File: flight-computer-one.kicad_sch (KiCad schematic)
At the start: 10 parts, among them J1 LEFT_BANK, J2 RIGHT_BANK

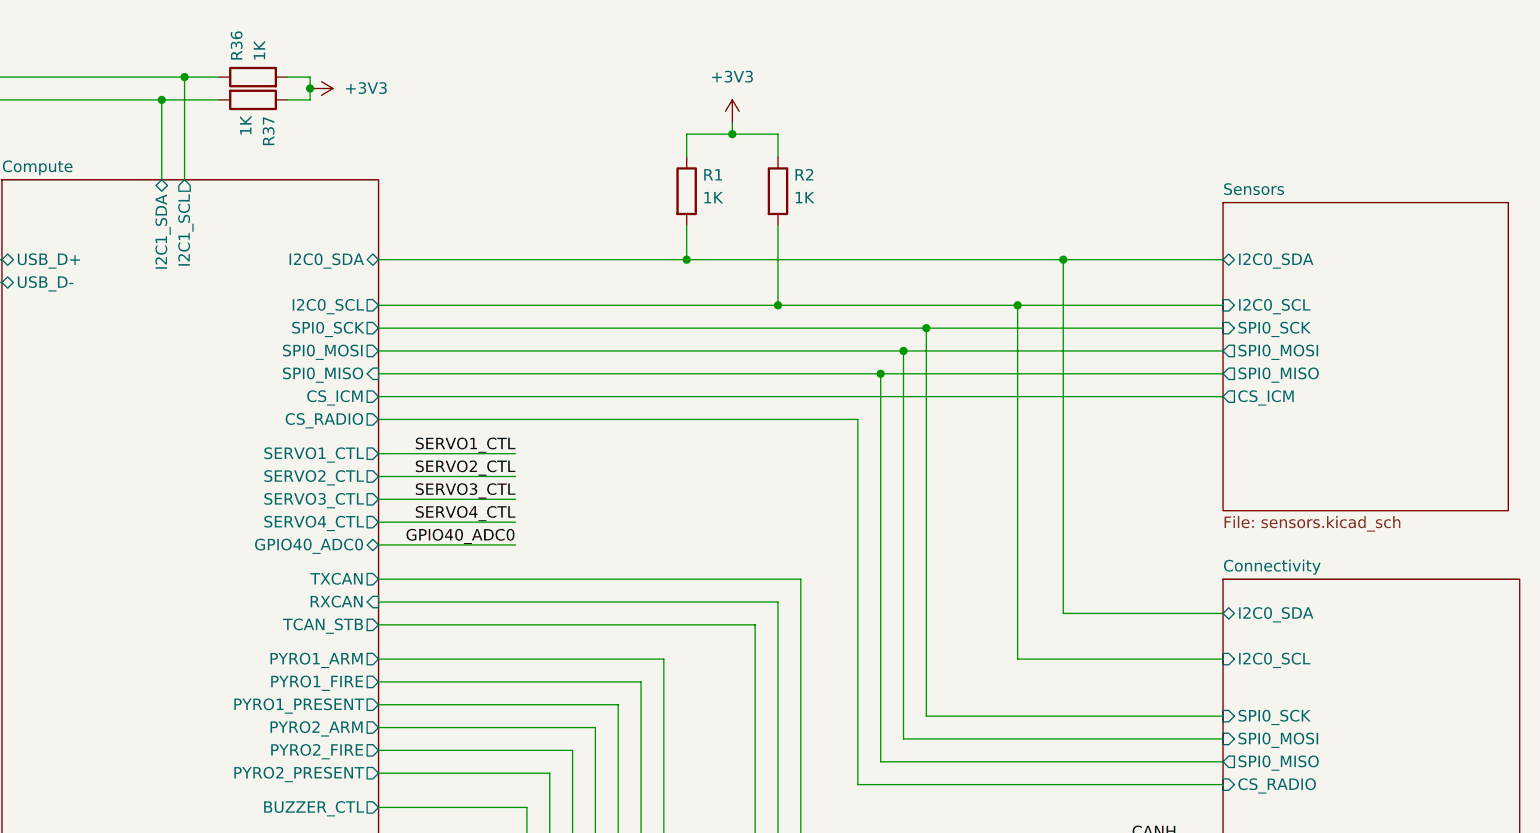
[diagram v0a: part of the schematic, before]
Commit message: new routing
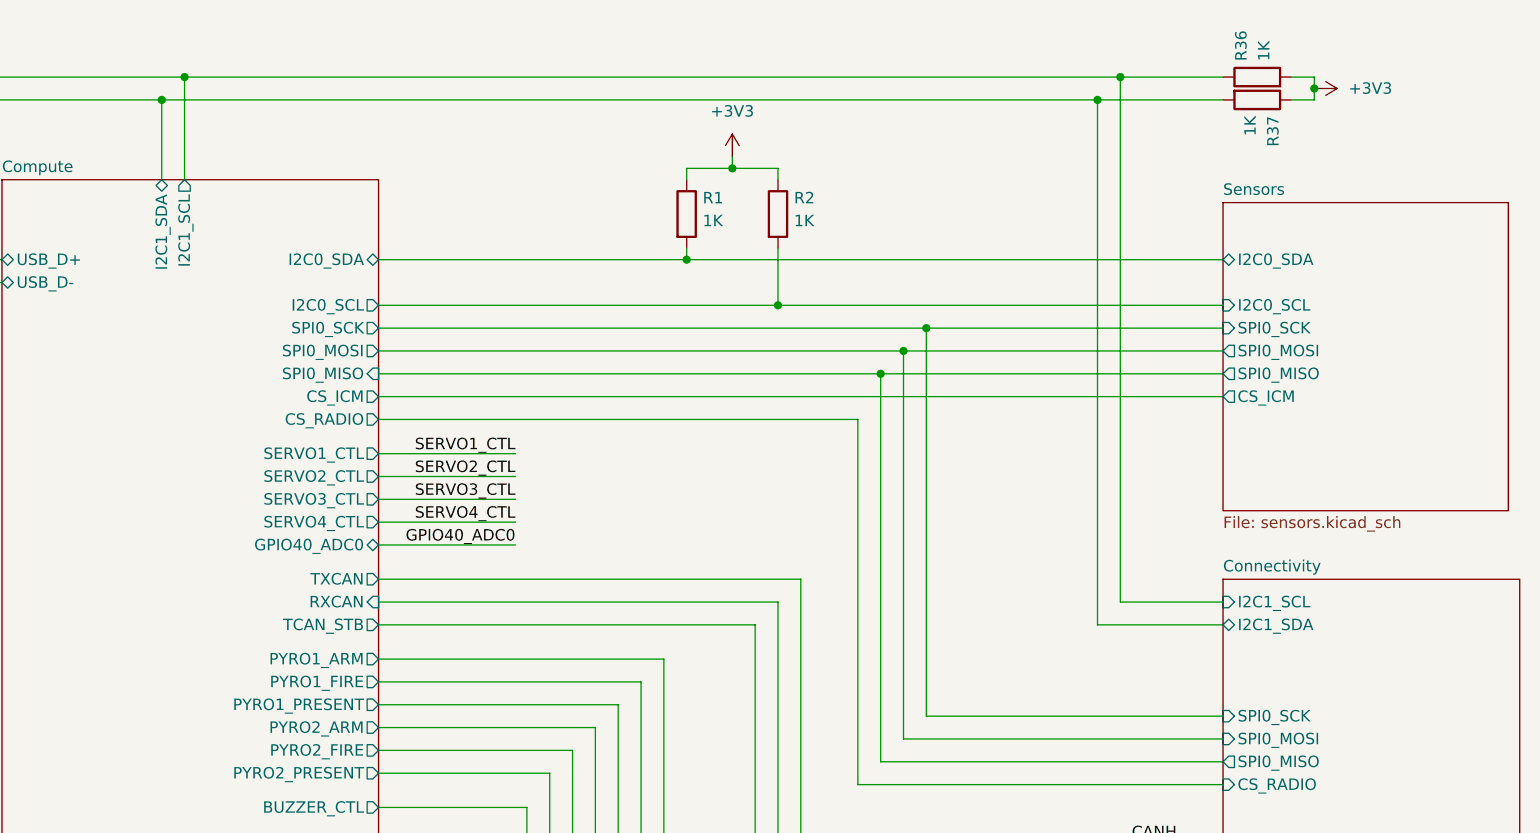
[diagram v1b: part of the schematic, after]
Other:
- sheet Connectivity ports: added I2C1_SCL, I2C1_SDA; removed I2C0_SCL, I2C0_SDA
- moved on the sheet: R1, R2, R36, R37

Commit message: final production files
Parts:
- J1, J2: DK Part (none) -> https://www.digikey.com/en/products/detail/amphenol-anytek/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
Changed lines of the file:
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@@
+			)
+		)
+		(property "DK Part" "https://www.digikey.com/en/products/detail/amphenol-anytek/VI0801550000G/2261365"
+			(at 91.44 147.32 0)
+			(effects
+				(font
+					(size 1.27 1.27)
+				)
+				(hide yes)
 			)
 		)
@@
 			(at 121.92 149.86 0)
 			(effects
+				(font
+					(size 1.27 1.27)
+				)
+				(hide yes)
+			)
+		)
+		(property "DK Part" "https://www.digikey.com/en/products/detail/amphenol-anytek/VI0801550000G/2261365"
+			(at 121.92 149.86 0)
+			(effects
